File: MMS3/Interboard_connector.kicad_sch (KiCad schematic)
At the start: 1 part, among them J1 86093488324755V1LF

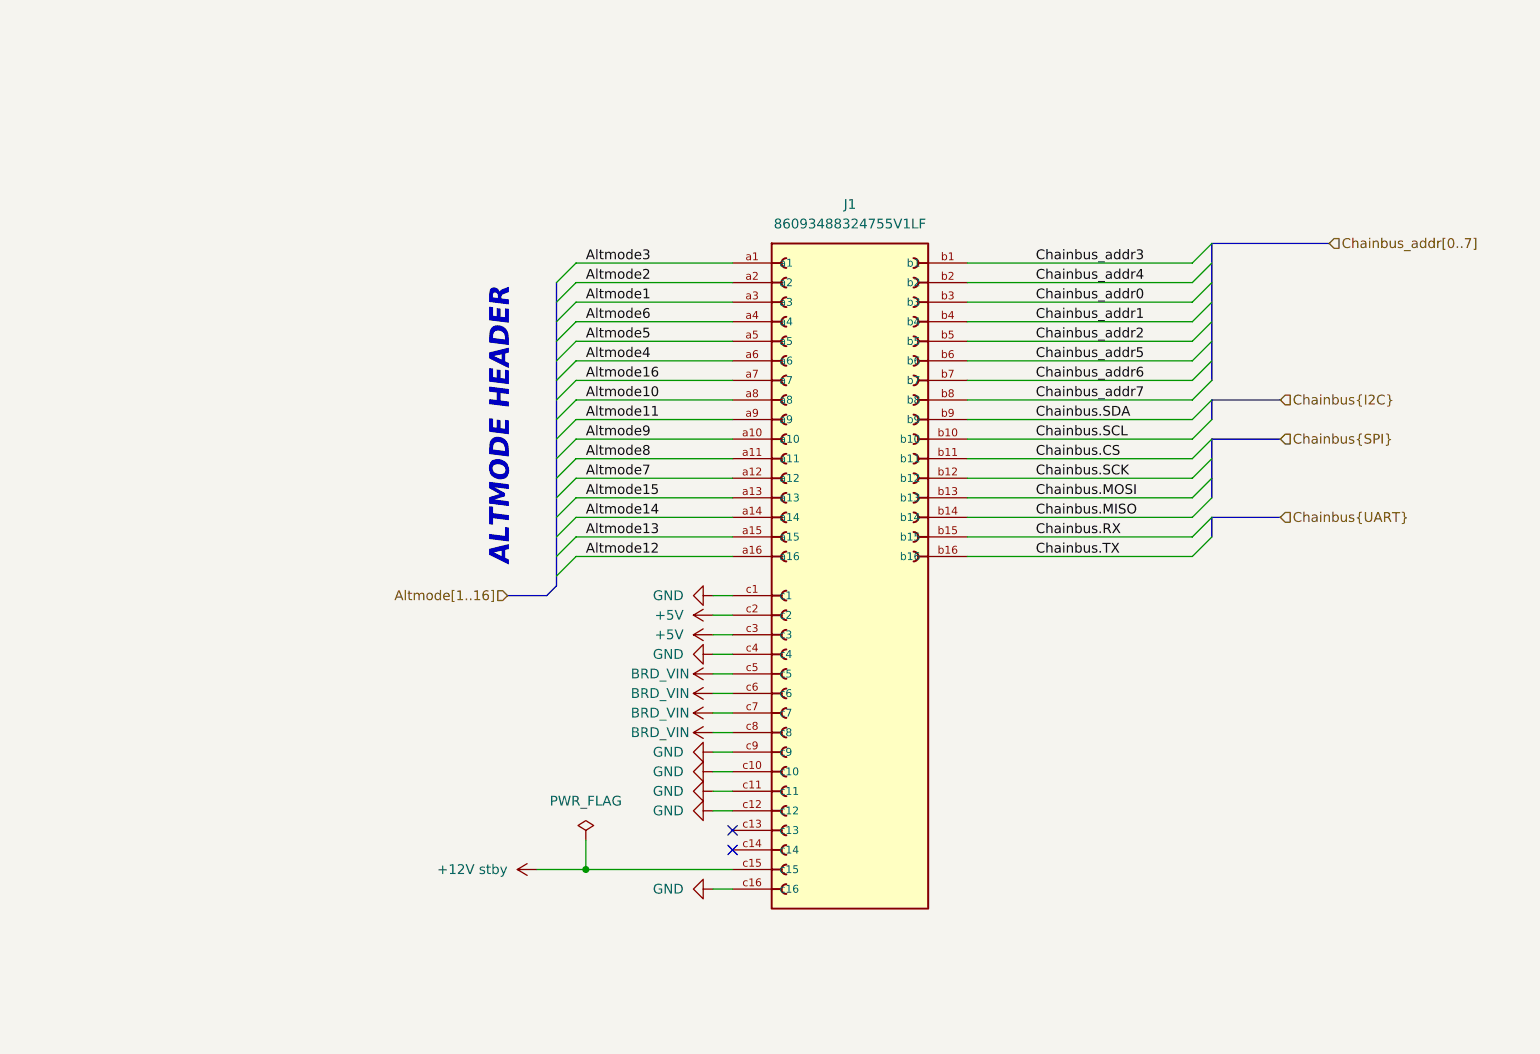
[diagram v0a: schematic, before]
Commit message: finished routing
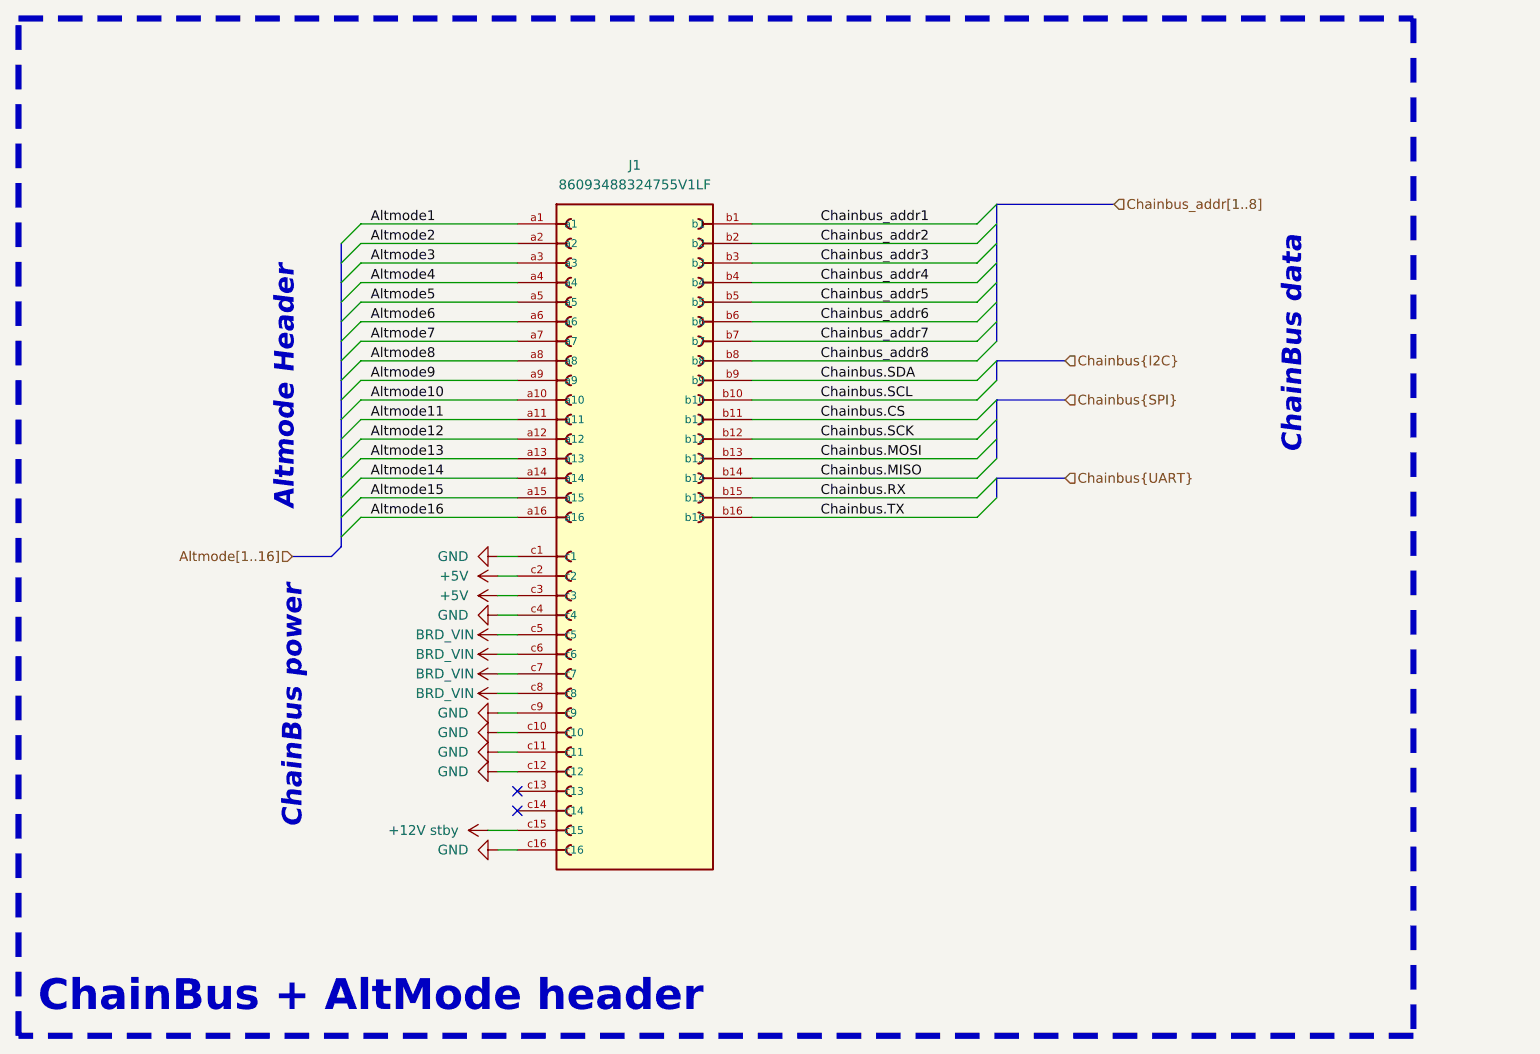
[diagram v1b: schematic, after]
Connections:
- net Chainbus_addr0 is gone; now on net Chainbus_addr3: J1.b3
- net Altmode1: now also J1.a1; no longer J1.a3
- net Altmode10: now also J1.a10; no longer J1.a8
- net Altmode11: now also J1.a11; no longer J1.a9
- net Altmode12: now also J1.a12; no longer J1.a16
- net Altmode13: now also J1.a13; no longer J1.a15
- net Altmode15: now also J1.a15; no longer J1.a13
- net Altmode16: now also J1.a16; no longer J1.a7
- net Altmode3: now also J1.a3; no longer J1.a1
- net Altmode4: now also J1.a4; no longer J1.a6
- net Altmode6: now also J1.a6; no longer J1.a4
- net Altmode7: now also J1.a7; no longer J1.a12
- net Altmode8: now also J1.a8; no longer J1.a11
- net Altmode9: now also J1.a9; no longer J1.a10
- net Chainbus_addr1: now also J1.b1; no longer J1.b4
- net Chainbus_addr2: now also J1.b2; no longer J1.b5
- net Chainbus_addr3: no longer J1.b1
- net Chainbus_addr4: now also J1.b4; no longer J1.b2
- net Chainbus_addr5: now also J1.b5; no longer J1.b6
- net Chainbus_addr6: now also J1.b6; no longer J1.b7
- net Chainbus_addr7: now also J1.b7; no longer J1.b8
- new net Chainbus_addr8: J1.b8
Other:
- note added: "Altmode Header"
- note added: "ChainBus + AltMode header"
- note added: "ChainBus data"
- note added: "ChainBus power"
- note removed: "ALTMODE HEADER"
- title: MMS3 -> MMS3 MCU ESP32-C6
- moved on the sheet: J1
